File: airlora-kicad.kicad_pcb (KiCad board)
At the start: 4 copper layers, 77 x 77 mm, 185 parts, among them IC1 BALFHB-WL-02D3, J1 12V, J10 I2C, J11 UART2, J12 UART_MAIN, J2 Conn_Coaxial, J3 Led, J4 SHT, J5 I2C, J6 A_NO2, J7 UART1, J8 A_CO, J9 I2C, Q1 S8050, Q2 S8050, Q3 S8050, Q4 S8050, Q5 S8050, Q6 S8050, Q7 S8050, Q8 S8050, Q9 S8050, SW1 SW_Push, SW2 SW_Slide_DPDT, SW3 SW_Push, U1 TPS7A2633DRVR, U2 TPS54202DDC, U3 TPS7A2633DRVR, U4 BGS12WN6E6327, U5 STM32WLE5CCUx, U6 STM32F103C8Tx, X1 32MHZ, Y1 32.768kHz, Y2 8Mhz

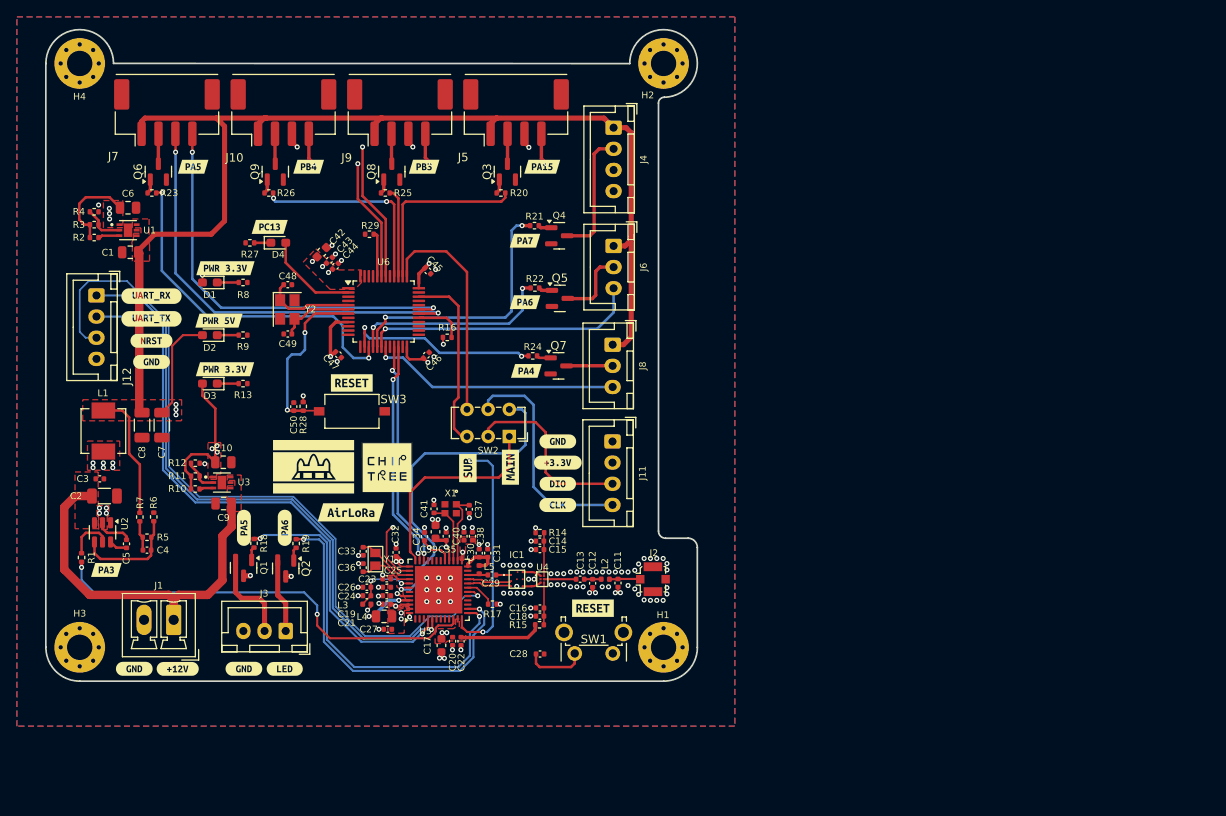
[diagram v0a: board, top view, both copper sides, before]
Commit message: Update PCB layout
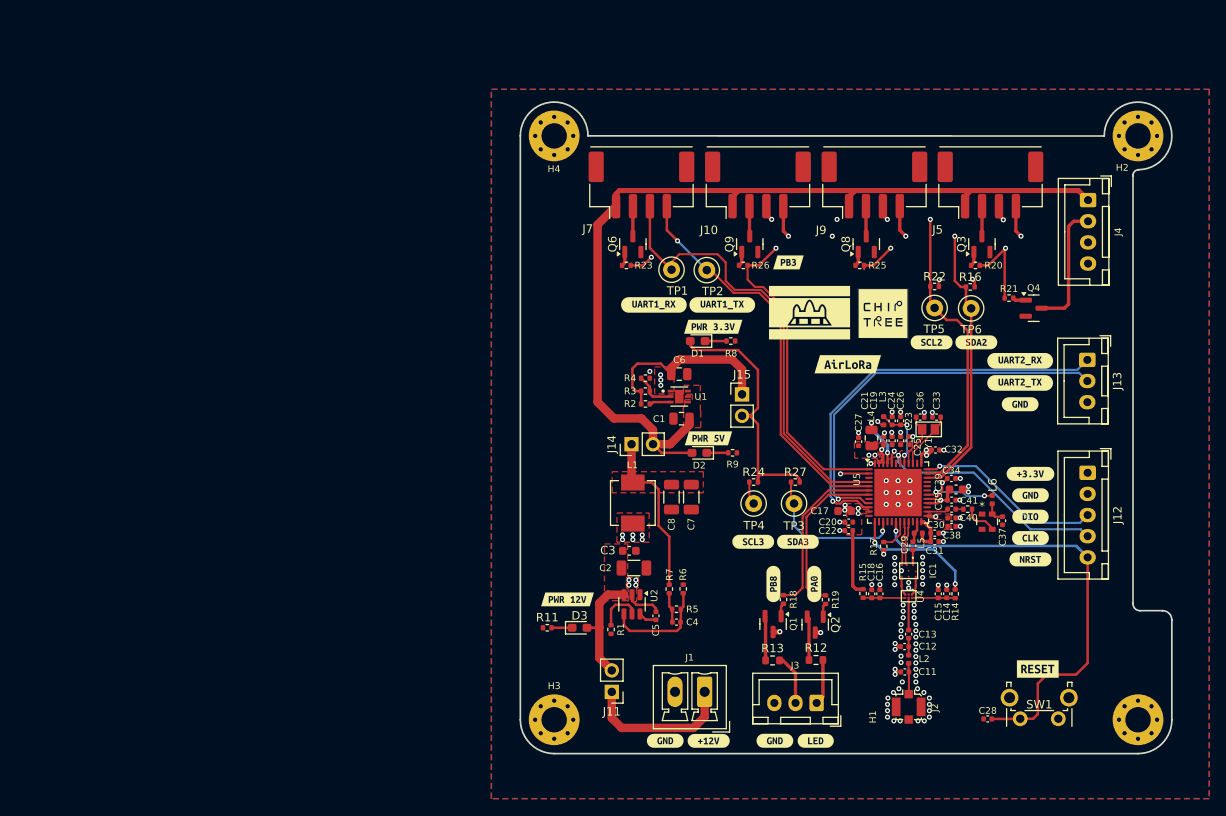
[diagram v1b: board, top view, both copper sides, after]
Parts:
- removed C10, C9: 1uF, Capacitor_SMD:C_0805_2012Metric
- removed C42: 4.7uF, Capacitor_SMD:C_0603_1608Metric
- removed C43, C44, C45, C46, C47: 100nf, Capacitor_SMD:C_0402_1005Metric
- removed C48, C49: 22PF, Capacitor_SMD:C_0402_1005Metric
- removed C50: 100nF, Capacitor_SMD:C_0402_1005Metric
- removed D4: LED, LED_SMD:LED_0603_1608Metric_Pad1.05x0.95mm_HandSolder
- removed J6: A_NO2, Connector_JST:JST_XH_B3B-XH-A_1x03_P2.50mm_Vertical
- removed J8: A_CO, Connector_JST:JST_XH_B3B-XH-A_1x03_P2.50mm_Vertical
- removed Q5, Q7: S8050, Package_TO_SOT_SMD:SOT-23
- removed R28, R29: 10k, Resistor_SMD:R_0402_1005Metric
- removed SW2: SW_Slide_DPDT, Button_Switch_THT:SW_E-Switch_EG1271_SPDT
- removed SW3: SW_Push, Button_Switch_SMD:SW_Tactile_SPST_NO_Straight_CK_PTS636Sx25SMTRLFS
- removed U3: TPS7A2633DRVR, footprint:TPS7A2633DRVR
- removed U6: STM32F103C8Tx, Package_QFP:LQFP-48_7x7mm_P0.5mm
- removed X1: 32MHZ, footprint:NX2016SA_NDK
- removed Y2: 8Mhz, Crystal:Crystal_SMD_3225-4Pin_3.2x2.5mm
- removed kibuzzard-667528BC: G***, kibuzzard-667528BC
- removed kibuzzard-667528D4: G***, kibuzzard-667528D4
- removed the kibuzzard-66752922 at (124.1, 87.6)
- removed the kibuzzard-66752922 at (123.9, 76.0)
- removed the kibuzzard-667540EB at (124.1, 85.1)
- removed the kibuzzard-667540EB at (123.9, 73.6)
- removed kibuzzard-66754104: G***, kibuzzard-66754104
- removed the kibuzzard-66754176 at (96.7, 89.6)
- removed kibuzzard-667541E6 (x4): G***, kibuzzard-667541E6
- removed kibuzzard-667541EF (x4): G***, kibuzzard-667541EF
- removed kibuzzard-66754524: G***, kibuzzard-66754524
- removed the kibuzzard-66763ACD at (81.7, 87.9)
- removed kibuzzard-668CA440: G***, kibuzzard-668CA440
- removed kibuzzard-668CA458: G***, kibuzzard-668CA458
- removed kibuzzard-668CA46A: G***, kibuzzard-668CA46A
- removed kibuzzard-668CA479: G***, kibuzzard-668CA479
- removed kibuzzard-668CA498: G***, kibuzzard-668CA498
- removed kibuzzard-668CA4A7: G***, kibuzzard-668CA4A7
- removed kibuzzard-668CA4B6: G***, kibuzzard-668CA4B6
- removed kibuzzard-668CA4DF: G***, kibuzzard-668CA4DF
- removed kibuzzard-668CA658: G***, kibuzzard-668CA658
- removed kibuzzard-668CA679: G***, kibuzzard-668CA679
- removed kibuzzard-668F38B2: G***, kibuzzard-668F38B2
- removed kibuzzard-6690D059: G***, kibuzzard-6690D059
- removed kibuzzard-6690D084: G***, kibuzzard-6690D084
- removed kibuzzard-6690D099: G***, kibuzzard-6690D099
- added J13: UART_MAIN, Connector_JST:JST_XH_B3B-XH-A_1x03_P2.50mm_Vertical, F.Cu at (183.6, 86.8)
- added J14: Conn_01x02_Pin, Connector_PinHeader_2.54mm:PinHeader_1x02_P2.54mm_Vertical, F.Cu at (129.7, 96.8)
- added J15: Conn_01x02_Pin, Connector_PinHeader_2.54mm:PinHeader_1x02_P2.54mm_Vertical, F.Cu at (142.8, 90.9)
- added L6: 1400R@1GHz, Inductor_SMD:L_0402_1005Metric, F.Cu at (172.4, 103.3)
- added TP1: TestPoint, TestPoint:TestPoint_Loop_D1.80mm_Drill1.0mm_Beaded, F.Cu at (134.5, 76.2)
- added TP2: TestPoint, TestPoint:TestPoint_Loop_D1.80mm_Drill1.0mm_Beaded, F.Cu at (138.6, 76.2)
- added TP3: TestPoint, TestPoint:TestPoint_Loop_D1.80mm_Drill1.0mm_Beaded, F.Cu at (149.0, 103.8)
- added TP4: TestPoint, TestPoint:TestPoint_Loop_D1.80mm_Drill1.0mm_Beaded, F.Cu at (144.2, 103.8)
- added TP5: TestPoint, TestPoint:TestPoint_Loop_D1.80mm_Drill1.0mm_Beaded, F.Cu at (165.6, 80.7)
- added TP6: TestPoint, TestPoint:TestPoint_Loop_D1.80mm_Drill1.0mm_Beaded, F.Cu at (169.9, 80.7)
- added XTAL1: NT2016SA-32M-END4263A, footprint:NT2016SA-32M-END4263A_NDK, F.Cu at (171.8, 105.9)
- added kibuzzard-66752922: G***, kibuzzard-66752922, F.Cu at (175.7, 92.1)
- added kibuzzard-66A47256: G***, kibuzzard-66A47256, F.Cu at (122.2, 115.1)
- added kibuzzard-66A70081: G***, kibuzzard-66A70081, B.Cu at (145.7, 63.9)
- added kibuzzard-66A7008A: G***, kibuzzard-66A7008A, B.Cu at (147.7, 63.9)
- added kibuzzard-66A70091: G***, kibuzzard-66A70091, B.Cu at (159.5, 64.0)
- added kibuzzard-66A70098: G***, kibuzzard-66A70098, B.Cu at (161.4, 64.0)
- added kibuzzard-66A700A1: G***, kibuzzard-66A700A1, B.Cu at (173.2, 64.1)
- added kibuzzard-66A704F7: G***, kibuzzard-66A704F7, B.Cu at (175.2, 64.1)
- added kibuzzard-66A704FE: G***, kibuzzard-66A704FE, F.Cu at (170.5, 84.8)
- added kibuzzard-66A704FE: G***, kibuzzard-66A704FE, B.Cu at (179.6, 75.3)
- added kibuzzard-66A70504: G***, kibuzzard-66A70504, F.Cu at (165.2, 84.8)
- added kibuzzard-66A70504: G***, kibuzzard-66A70504, B.Cu at (179.6, 72.8)
- added kibuzzard-66A7052C: G***, kibuzzard-66A7052C, F.Cu at (132.4, 80.3)
- added kibuzzard-66A70534: G***, kibuzzard-66A70534, F.Cu at (140.5, 80.3)
- added kibuzzard-66A705CB: G***, kibuzzard-66A705CB, F.Cu at (149.4, 108.3)
- added kibuzzard-66A705D3: G***, kibuzzard-66A705D3, F.Cu at (144.1, 108.3)
- added kibuzzard-66A7121E: G***, kibuzzard-66A7121E, F.Cu at (175.7, 86.9)
- added kibuzzard-66A71226: G***, kibuzzard-66A71226, F.Cu at (175.7, 89.5)
- added kibuzzard-66A7130C: G***, kibuzzard-66A7130C, F.Cu at (146.5, 113.3)
- added kibuzzard-66A71314: G***, kibuzzard-66A71314, F.Cu at (151.3, 113.3)
- added kibuzzard-66A71938: G***, kibuzzard-66A71938, F.Cu at (148.3, 75.3)
- C3: footprint Capacitor_SMD:C_0402_1005Metric -> Capacitor_SMD:C_0603_1608Metric
- C37, C41: value 6.8pF -> 10pF
- J11: value UART2 -> Conn_01x02_Pin; footprint Connector_JST:JST_XH_B4B-XH-A_1x04_P2.50mm_Vertical -> Connector_PinHeader_2.54mm:PinHeader_1x02_P2.54mm_Vertical
- J12: value UART_MAIN -> STlink; footprint Connector_JST:JST_XH_B4B-XH-A_1x04_P2.50mm_Vertical -> Connector_JST:JST_XH_B5B-XH-A_1x05_P2.50mm_Vertical
- R10: value 10K -> 220
- R11: value 1.96M -> 3k
- R12: value 1.18M -> 1K; footprint Resistor_SMD:R_0402_1005Metric -> Resistor_SMD:R_0603_1608Metric
- R13: value 1k -> 1K; footprint Resistor_SMD:R_0402_1005Metric -> Resistor_SMD:R_0603_1608Metric
- R16, R22, R24: value 1K -> 4.7K
- R27: value 1k -> 4.7K
- moved J12 119.0 mm to (183.6, 100.2)
- moved kibuzzard-6690D08F 107.0 mm to (176.9, 110.4)
- moved R10 91.3 mm to (169.5, 104.5)
- moved R12 76.9 mm to (151.5, 122.3)
- moved R13 70.6 mm to (146.4, 122.3)
- moved R27 70.4 mm to (149.1, 101.3), turned to 0 degrees
- moved C33 69.6 mm to (165.8, 93.6), turned to 180 degrees
- moved C36 68.2 mm to (163.9, 93.6), turned to 180 degrees
- moved C6 68.0 mm to (135.4, 88.5)
- moved U1 68.0 mm to (135.4, 91.2)
- moved C1 68.0 mm to (135.6, 93.8)
- moved R2 68.0 mm to (131.4, 92.0)
- moved R3 68.0 mm to (131.4, 90.5)
- moved R4 68.0 mm to (131.4, 89.0)
- moved Y1 67.1 mm to (164.8, 95.0), turned to 0 degrees
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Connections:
- C29 pad 2: /AirLora V3/MCU/RFO_LP -> /AirLora V3/MCU/RFO_HP
- C37 pad 1: GND -> Net-(XTAL1-VCC)
- C37 pad 2: Net-(U5-OSC_IN) -> GND
- C41 pad 1: Net-(U5-OSC_OUT) -> /AirLora V3/MCU/XTA
- C41 pad 2: GND -> Net-(C41-Pad2)
- C6 pad 1: +3.3V_HP -> Net-(J15-Pin_1)
- C7 pad 1: +5V -> a
- C8 pad 1: +5V -> a
- D1 pad 2: +3.3V_HP -> +3.3V
- D3 pad 2: +3.3V -> +12V
- J1 pad 1: +12V -> Net-(J1-Pin_1)
- J10 pad 3: /AirLora V3/MCU Sub/SCL1 -> /AirLora V3/MCU/SCL2
- J10 pad 4: /AirLora V3/MCU Sub/SDA1 -> /AirLora V3/MCU/SDA2
- J11 pad 1: GND -> Net-(J1-Pin_1)
- J11 pad 2: +3.3V -> +12V
- J12 pad 1: /AirLora V3/MCU/UART1_RX -> +3.3V
- J12 pad 2: /AirLora V3/MCU/UART1_TX -> GND
- J12 pad 3: /AirLora V3/MCU/NRST -> /AirLora V3/MCU/T_SWDIO
- J12 pad 4: GND -> /AirLora V3/MCU/T_SWCLK
- J4 pad 3: /AirLora V3/MCU Sub/SCL1 -> /AirLora V3/MCU/SCL2
- J4 pad 4: /AirLora V3/MCU Sub/SDA1 -> /AirLora V3/MCU/SDA2
- J5 pad 3: /AirLora V3/MCU Sub/SCL1 -> /AirLora V3/MCU/SCL2
- J5 pad 4: /AirLora V3/MCU Sub/SDA1 -> /AirLora V3/MCU/SDA2
- J7 pad 3: /AirLora V3/MCU Sub/TX3 -> /AirLora V3/MCU/UART1_TX
- J7 pad 4: /AirLora V3/MCU Sub/RX3 -> /AirLora V3/MCU/UART1_RX
- J9 pad 3: /AirLora V3/MCU Sub/SCL1 -> /AirLora V3/MCU/SCL2
- J9 pad 4: /AirLora V3/MCU Sub/SDA1 -> /AirLora V3/MCU/SDA2
- L1 pad 2: +5V -> a
- L5 pad 2: /AirLora V3/MCU/RFO_LP -> /AirLora V3/MCU/RFO_HP
- Q1 pad 2: Net-(J3-Pin_2) -> Net-(Q1-E)
- Q2 pad 2: Net-(J3-Pin_1) -> Net-(Q2-E)
- R1 pad 2: /AirLora V3/MCU/PA3 -> /AirLora V3/Power/En
- R10 pad 2: +3.3V -> Net-(C41-Pad2)
- R11 pad 1: +3.3V -> Net-(D3-K)
- R11 pad 2: Net-(U3-NC) -> GND
- R12 pad 1: Net-(U3-NC) -> Net-(Q2-E)
- R12 pad 2: GND -> Net-(J3-Pin_1)
- R13 pad 1: Net-(D3-K) -> Net-(Q1-E)
- R13 pad 2: GND -> Net-(J3-Pin_2)
- R16 pad 1: Net-(U5-PA4) -> /AirLora V3/MCU/SDA2
- R16 pad 2: /AirLora V3/MCU Sub/PA8 -> +3.3V
- R18 pad 1: /AirLora V3/MCU/PA5 -> /AirLora V3/MCU/PB8
- R19 pad 1: /AirLora V3/MCU/PA6 -> /AirLora V3/MCU/PA0
- R2 pad 2: +3.3V_HP -> Net-(J15-Pin_1)
- R20 pad 1: /AirLora V3/MCU Sub/PA15 -> /AirLora V3/MCU/PB3
- R21 pad 2: /AirLora V3/MCU Sub/PA7 -> /AirLora V3/MCU/PB3
- R22 pad 1: /AirLora V3/MCU Sub/PA6 -> /AirLora V3/MCU/SCL2
- R22 pad 2: Net-(Q5-B) -> +3.3V
- R23 pad 1: /AirLora V3/MCU Sub/PA5 -> /AirLora V3/MCU/PB3
- R24 pad 1: /AirLora V3/MCU Sub/PA4 -> /AirLora V3/MCU/SDA3
- R24 pad 2: Net-(Q7-B) -> +3.3V
- R25 pad 1: /AirLora V3/MCU Sub/PB3 -> /AirLora V3/MCU/PB3
- R26 pad 1: /AirLora V3/MCU Sub/PB4 -> /AirLora V3/MCU/PB3
- R27 pad 1: Net-(D4-K) -> /AirLora V3/MCU/SCL3
- R27 pad 2: GND -> +3.3V
- R3 pad 1: +3.3V_HP -> Net-(J15-Pin_1)
- R7 pad 2: +5V -> a
- U1 pad 1: +3.3V_HP -> Net-(J15-Pin_1)
- U5 pad 1: unconnected-(U5-PB3-Pad1) -> /AirLora V3/MCU/PB3
- U5 pad 10: /AirLora V3/MCU/PA3 -> /AirLora V3/MCU/UART2_RX
- U5 pad 12: Net-(U5-PA4) -> unconnected-(U5-PA4-Pad12)
- U5 pad 13: /AirLora V3/MCU/PA5 -> /AirLora V3/MCU/FE_CTRL1
- U5 pad 14: /AirLora V3/MCU/PA6 -> unconnected-(U5-PA6-Pad14)
- U5 pad 15: unconnected-(U5-PA7-Pad15) -> /AirLora V3/MCU/SCL3
- U5 pad 2: unconnected-(U5-PB4-Pad2) -> /AirLora V3/MCU/SDA3
- U5 pad 22: /AirLora V3/MCU/RFO_LP -> unconnected-(U5-RFO_LP-Pad22)
- U5 pad 23: unconnected-(U5-RFO_HP-Pad23) -> /AirLora V3/MCU/RFO_HP
- U5 pad 26: Net-(U5-OSC_IN) -> /AirLora V3/MCU/XTA
- U5 pad 27: Net-(U5-OSC_OUT) -> unconnected-(U5-OSC_OUT-Pad27)
- U5 pad 30: unconnected-(U5-PB0-VDD_TCXO-Pad30) -> /AirLora V3/MCU/PB0
- U5 pad 34: /AirLora V3/MCU Sub/SCL2 -> /AirLora V3/MCU/SDA2
- U5 pad 35: /AirLora V3/MCU Sub/SDA2 -> /AirLora V3/MCU/SCL2
- U5 pad 38: /AirLora V3/MCU/FE_CTRL1 -> unconnected-(U5-PC13-Pad38)
- U5 pad 6: unconnected-(U5-PB8-Pad6) -> /AirLora V3/MCU/PB8
- U5 pad 7: unconnected-(U5-PA0-Pad7) -> /AirLora V3/MCU/PA0
- U5 pad 9: unconnected-(U5-PA2-Pad9) -> /AirLora V3/MCU/UART2_TX
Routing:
- net /AirLora V3/MCU/PB3: track 0.00 -> 97.3 mm, vias 0 -> 4
- net /AirLora V3/MCU/SDA2: track 0.00 -> 81.1 mm, vias 0 -> 5
- net /AirLora V3/MCU/SCL2: track 0.00 -> 79.4 mm, vias 0 -> 5
- net /AirLora V3/MCU Sub/SDA1: track 62.6 -> 0.00 mm, vias 4 -> 0
- net /AirLora V3/MCU Sub/SCL1: track 60.4 -> 0.00 mm, vias 4 -> 0
- net /AirLora V3/MCU/NRST: track 114.6 -> 54.3 mm
- net +5V: track 169.6 -> 111.0 mm, vias 5 -> 2
- net /AirLora V3/MCU/PA3: track 51.9 -> 0.00 mm, vias 2 -> 0
- net /AirLora V3/MCU Sub/TX3: track 51.8 -> 0.00 mm, vias 2 -> 0
- net /AirLora V3/MCU Sub/RX3: track 48.9 -> 0.00 mm, vias 2 -> 0
- net /AirLora V3/MCU/UART2_RX: track 0.00 -> 48.3 mm, vias 0 -> 1
- net /AirLora V3/MCU/UART2_TX: track 0.00 -> 46.5 mm, vias 0 -> 1
- net /AirLora V3/MCU/PA5: track 46.1 -> 0.00 mm, vias 2 -> 0
- net Net-(U5-PA4): track 44.3 -> 0.00 mm, vias 3 -> 0
- net /AirLora V3/MCU/PA6: track 42.7 -> 0.00 mm, vias 2 -> 0
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- added copper zone on F.Cu, net Net-(J15-Pin_1)
- added copper zone on F.Cu, net a
- removed copper zone on F.Cu, net +3.3V_HP
- removed copper zone on In2.Cu, net +3.3V_HP
